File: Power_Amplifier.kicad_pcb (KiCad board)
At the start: 2 copper layers, 57 x 27.9 mm, 21 parts, among them Q1 BC547, Q2 2N3904

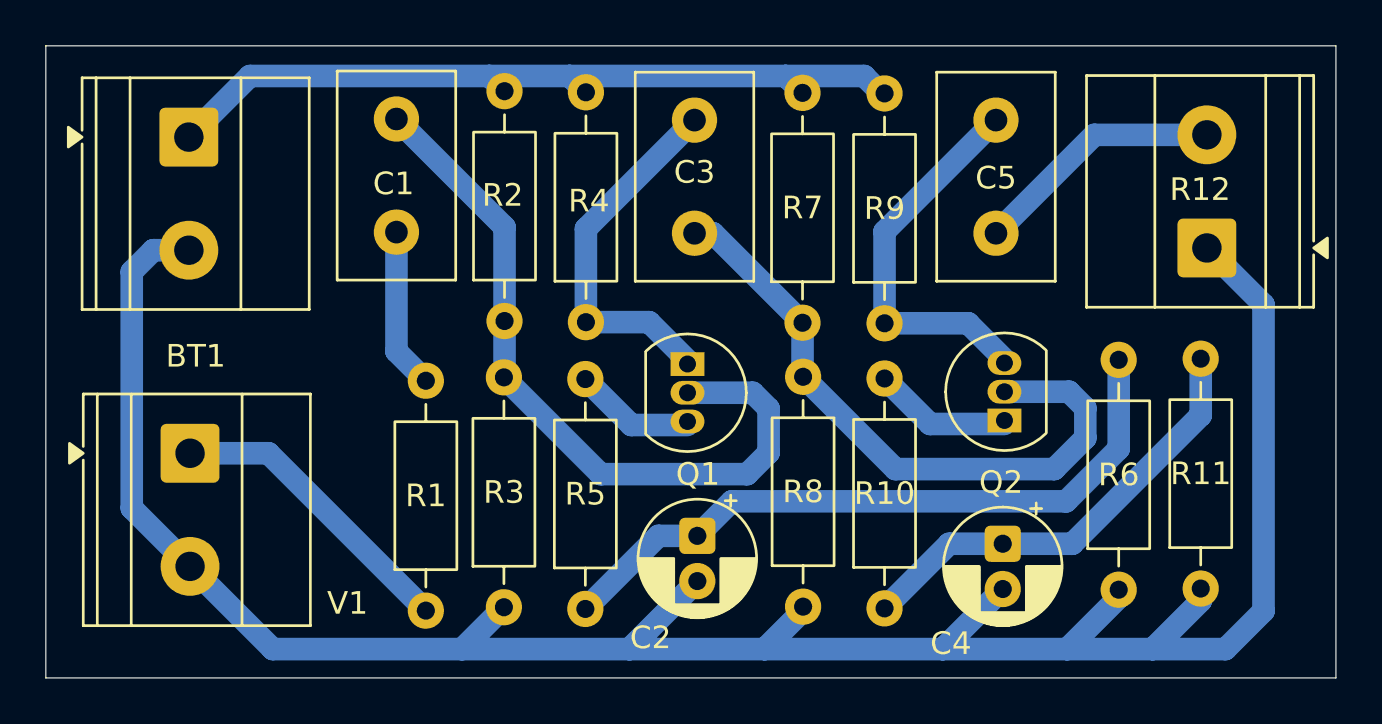
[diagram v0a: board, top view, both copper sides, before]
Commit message: version 1.1: 2.26.2026
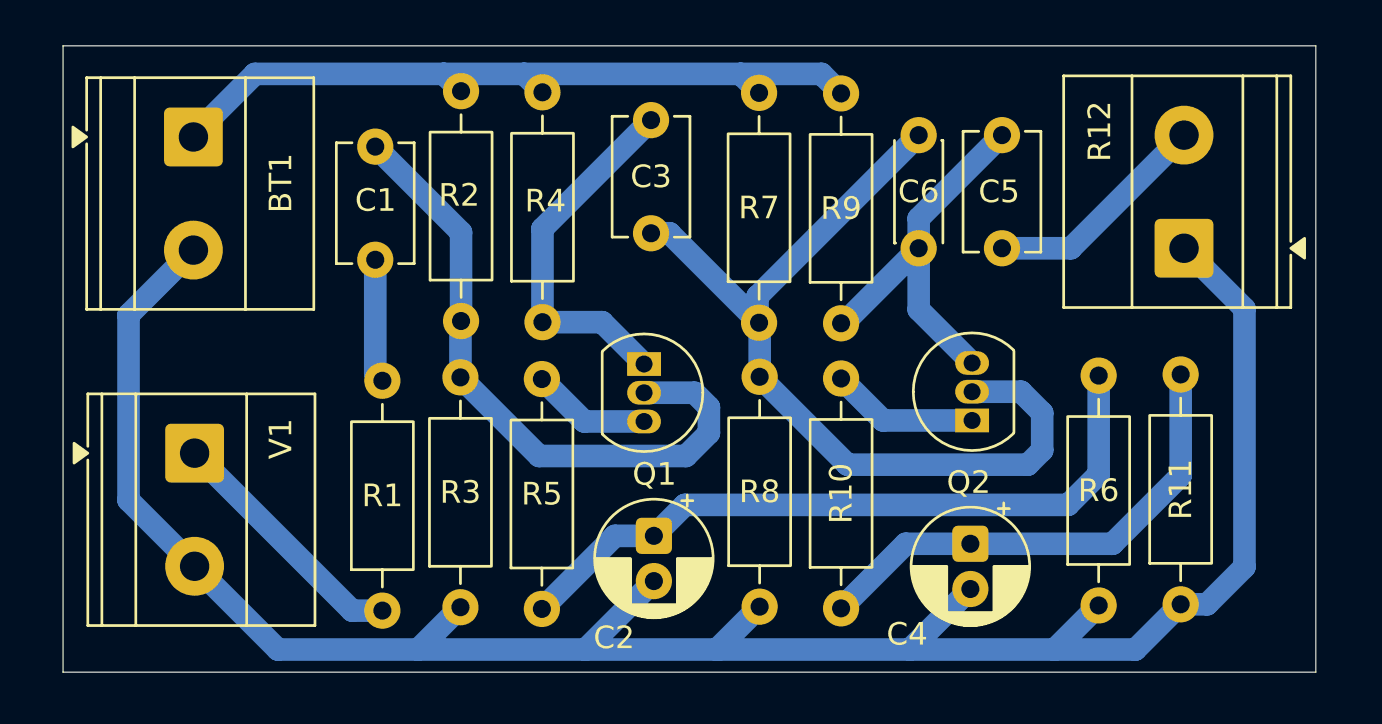
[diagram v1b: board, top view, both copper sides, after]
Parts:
- added C6: 180 uF, Capacitor_THT:C_Disc_D4.3mm_W1.9mm_P5.00mm, F.Cu at (108.8, 58.4)
- C1, C3, C5: footprint Capacitor_THT:C_Disc_D9.0mm_W5.0mm_P5.00mm -> Capacitor_THT:C_Disc_D5.1mm_W3.2mm_P5.00mm
- moved R10 1.92 mm to (105.4, 74.3)
- moved R2 1.92 mm to (88.6, 61.6)
- moved R3 1.92 mm to (88.6, 74.2)
- moved R4 1.92 mm to (92.2, 61.6)
- moved R7 1.92 mm to (101.8, 61.7)
- moved R9 1.92 mm to (105.4, 61.7)
- moved C2 1.92 mm to (97.1, 71.1)
- moved C3 1.92 mm to (97.0, 52.7)
- moved Q1 1.92 mm to (96.7, 63.5)
- moved R1 1.92 mm to (85.1, 74.4)
- moved R5 1.92 mm to (92.2, 74.3)
- moved R8 1.92 mm to (101.8, 74.2)
- moved C1 1.54 mm to (84.8, 58.9)
- moved C4 1.43 mm to (111.1, 71.4)
- moved Q2 1.43 mm to (111.2, 66.0)
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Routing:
- net Net-(Q2-B): track 28.7 -> 39.6 mm
- net GND: track 104.1 -> 97.1 mm
- net Net-(Q1-B): track 33.1 -> 28.9 mm
- net Net-(R1-Pad1): track 13.3 -> 11.2 mm
- net Net-(C4-Pad1): track 20.0 -> 21.9 mm
- net Net-(C1-Pad1): track 7.11 -> 5.48 mm
- net Net-(BT1-+): track 35.2 -> 33.6 mm
- net Net-(C5-Pad1): track 11.1 -> 10.1 mm
- net Net-(C2-Pad1): track 30.4 -> 31.4 mm
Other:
- board size 57 x 27.9 mm -> 55.4 x 27.7 mm
